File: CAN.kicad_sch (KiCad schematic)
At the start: 6 parts, among them IC2 ADM3054, U2 AP1117-50

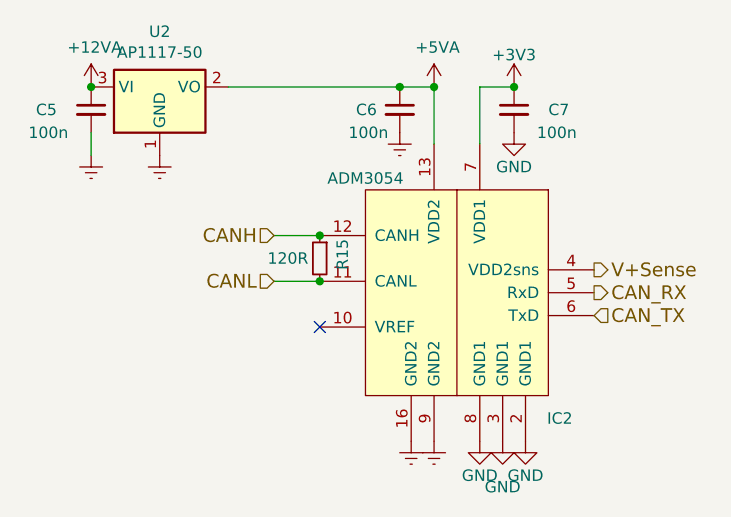
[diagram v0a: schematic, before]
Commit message: - some layout work
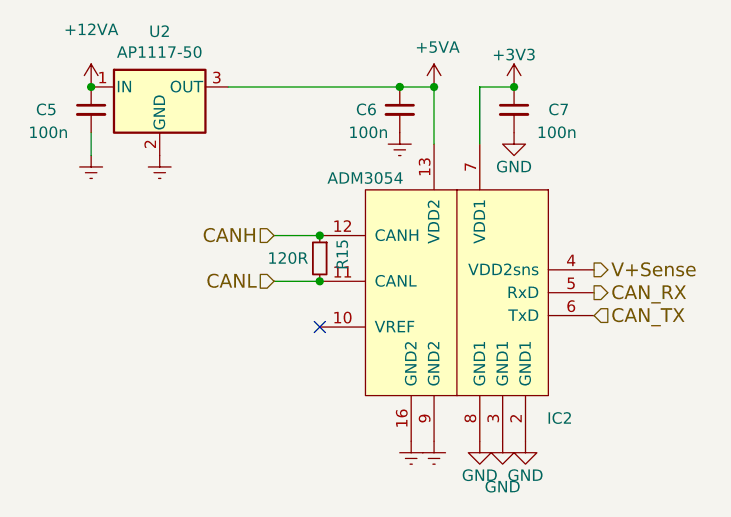
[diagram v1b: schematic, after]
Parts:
- U2: symbol Regulator_Linear:AP1117-50 -> Regulator_Linear:L7805
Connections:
- net +12VA: now also U2.1 (IN); no longer U2.3 (VI)
- net +5VA: now also U2.3 (OUT); no longer U2.2 (VO)
- net Earth: now also U2.2 (GND); no longer U2.1 (GND)
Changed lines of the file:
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@@
       (effects (font (size 1.27 1.27)) hide)
     )
-    (property "Value" "+12VA" (at 110.871 59.1058 0)
+    (property "Value" "+12VA" (at 110.49 57.15 0)
       (effects (font (size 1.27 1.27)))
     )
@@
     )
   )
-  (symbol (lib_id "Regulator_Linear:AP1117-50") (at 118.11 63.5 0) (unit 1)
+  (symbol (lib_id "Regulator_Linear:L7805") (at 118.11 63.5 0) (unit 1)
     (in_bom yes) (on_board yes) (dnp no)
     (property "Reference" "U2" (at 118.11 57.3532 0)
@@
       (effects (font (size 1.27 1.27)))
     )
-    (property "Footprint" "Package_TO_SOT_SMD:SOT-223-3_TabPin2" (at 118.11 58.42 0)
-      (effects (font (size 1.27 1.27)) hide)
-    )
-    (property "Datasheet" "http://www.diodes.com/datasheets/AP1117.pdf" (at 120.65 69.85 0)
-      (effects (font (size 1.27 1.27)) hide)
-    )
+    (property "Footprint" "Package_TO_SOT_SMD:SOT-223-3_TabPin2" (at 118.745 67.31 0)
+      (effects (font (size 1.27 1.27) italic) (justify left) hide)
+    )
+    (property "Datasheet" "http://www.st.com/content/ccc/resource/technical/document/datasheet/41/4f/b3/b0/12/d4/47/88/CD00000444.pdf/files/CD00000444.pdf/jcr:content/translations/en.CD00000444.pdf" (at 118.11 64.77 0)
+      (effects (font (size 1.27 1.27)) hide)
+    )
